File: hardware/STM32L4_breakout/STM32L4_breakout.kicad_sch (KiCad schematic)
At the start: 67 parts, among them J1 12V IN, J10 GPIO, J11 SPI1, J12 USART1, J13 USART3, J14 UART4, J15 3.3V, J16 5V, J17 12V, J2 SWD, J3 Conn_01x08, J4 Conn_01x06, J5 Conn_01x10, J6 Conn_01x08, J7 I2C1, J8 I2C2, J9 I2C3, SW1 SW_SPDT, U1 LD1117S50TR_SOT223, U2 LD3985M33R_SOT23, U3 LD1117S33TR_SOT223, U4 STM32L476RGTx, X1 NX3215SA-32.768K

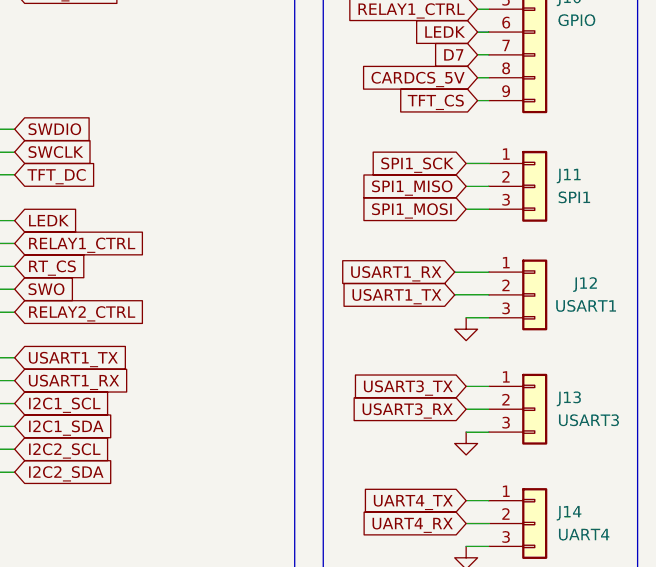
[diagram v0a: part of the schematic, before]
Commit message: breakout board signal routing WIP
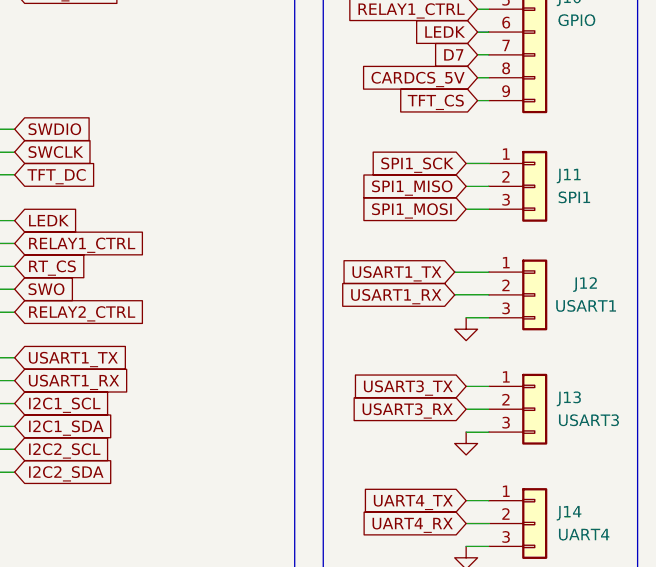
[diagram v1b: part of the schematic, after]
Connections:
- net USART1_RX: now also J12.2 (Pin_2); no longer J12.1 (Pin_1)
- net USART1_TX: now also J12.1 (Pin_1); no longer J12.2 (Pin_2)
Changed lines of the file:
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@@
-    (stroke (width 0) (type default) (color 0 0 0 0))
-  )
-  (wire (pts (xy 264.795 103.505) (xy 260.985 103.505))
     (stroke (width 0) (type default) (color 0 0 0 0))
   )
@@
     (stroke (width 0) (type default) (color 0 0 0 0))
   )
-  (wire (pts (xy 264.795 100.965) (xy 260.985 100.965))
-    (stroke (width 0) (type default) (color 0 0 0 0))
-  )
   (wire (pts (xy 62.865 178.435) (xy 66.04 178.435))
     (stroke (width 0) (type default) (color 0 0 0 0))
@@
     (stroke (width 0) (type default) (color 0 0 0 0))
   )
+  (wire (pts (xy 260.985 100.965) (xy 264.795 100.965))
+    (stroke (width 0) (type default) (color 0 0 0 0))
+  )
   (polyline (pts (xy 104.775 193.675) (xy 174.625 193.675))
     (stroke (width 0) (type default) (color 0 0 0 0))
@@
   )
   (wire (pts (xy 207.01 62.23) (xy 212.09 62.23))
+    (stroke (width 0) (type default) (color 0 0 0 0))
+  )
+  (wire (pts (xy 260.985 103.505) (xy 264.795 103.505))
     (stroke (width 0) (type default) (color 0 0 0 0))
   )
@@
     )
   )
-  (global_label "USART1_TX" (shape input) (at 260.985 103.505 180) (fields_autoplaced)
-    (effects (font (size 1.27 1.27)) (justify right))
-    (property "Intersheet References" "${INTERSHEET_REFS}" (id 0) (at 248.3514 103.4256 0)
+  (global_label "USART1_TX" (shape input) (at 260.985 100.965 180) (fields_autoplaced)
+    (effects (font (size 1.27 1.27)) (justify right))
+    (property "Intersheet References" "${INTERSHEET_REFS}" (id 0) (at 248.3514 100.8856 0)
       (effects (font (size 1.27 1.27)) (justify right) hide)
     )
@@
     )
   )
-  (global_label "USART1_RX" (shape input) (at 260.985 100.965 180) (fields_autoplaced)
-    (effects (font (size 1.27 1.27)) (justify right))
-    (property "Intersheet References" "${INTERSHEET_REFS}" (id 0) (at 248.049 100.8856 0)
-      (effects (font (size 1.27 1.27)) (justify right) hide)
-    )
+  (global_label "USART1_RX" (shape input) (at 260.985 103.505 180) (fields_autoplaced)
+    (effects (font (size 1.27 1.27)) (justify right))
+    (property "Intersheet References" "${INTERSHEET_REFS}" (id 0) (at 248.049 103.4256 0)
+      (effects (font (size 1.27 1.27)) (justify right) hide)
+    )
